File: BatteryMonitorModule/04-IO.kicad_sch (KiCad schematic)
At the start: 29 parts, among them J10 J_DISP_SPI, J11 J_UART, J12 J_EXP_B, J13 J_EXP_A, J5 J_FAN, J6 J_FAN_SEL, J7 J_NFC, J8 J_PANEL, Q5 2N7002

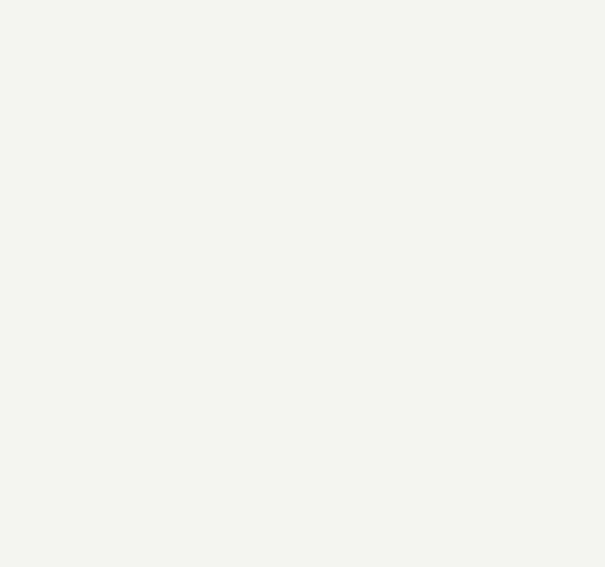
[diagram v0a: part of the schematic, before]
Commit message: design done commit
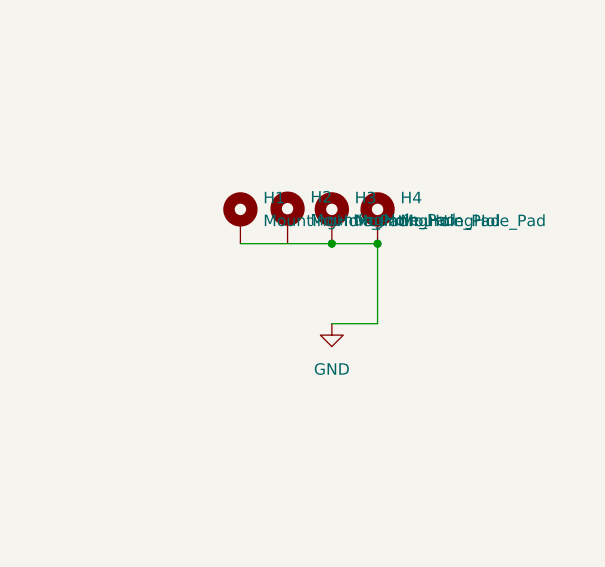
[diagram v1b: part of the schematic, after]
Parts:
- added H1, H2, H3, H4: MountingHole_Pad, symbol Mechanical:MountingHole_Pad
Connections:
- net GND: now also H1.1, H3.1, H4.1
